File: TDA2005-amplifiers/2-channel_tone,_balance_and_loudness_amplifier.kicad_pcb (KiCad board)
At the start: 2 copper layers, 38 parts, among them U1 TDA2005

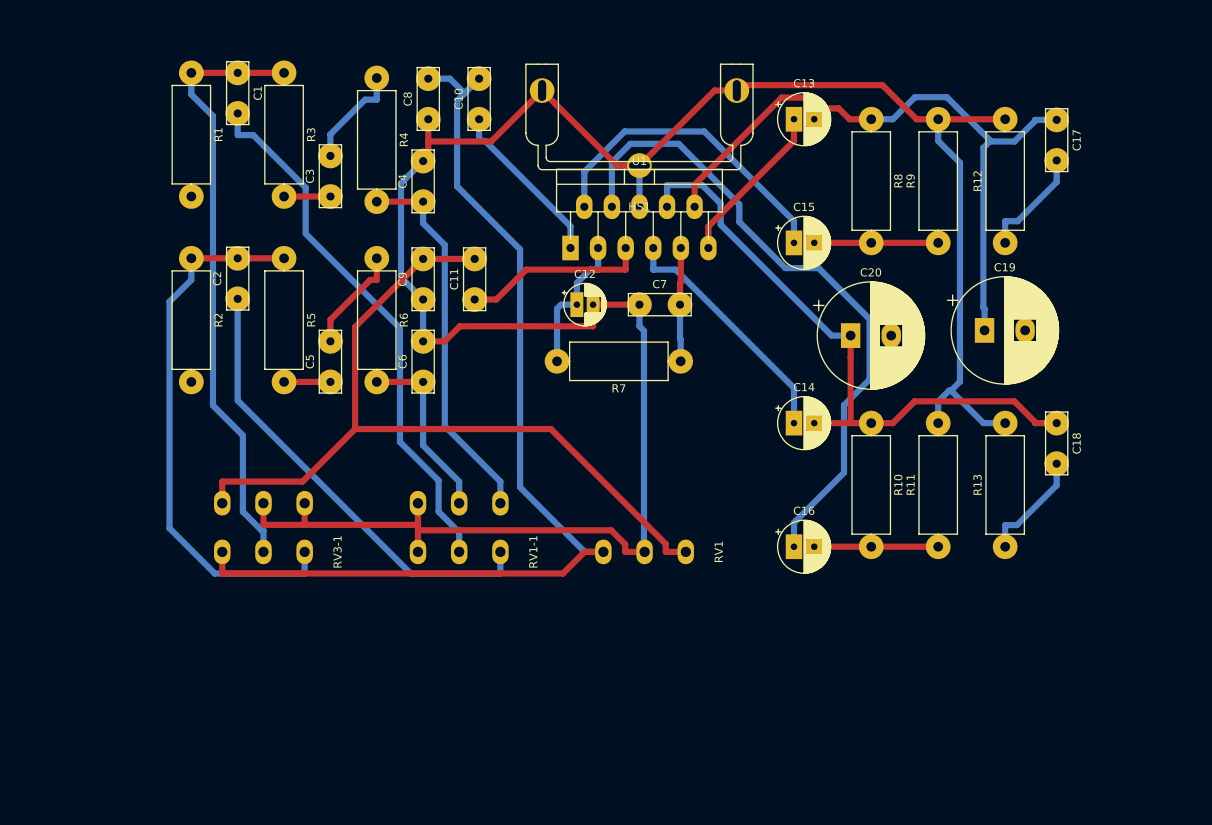
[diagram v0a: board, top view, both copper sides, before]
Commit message: new layout
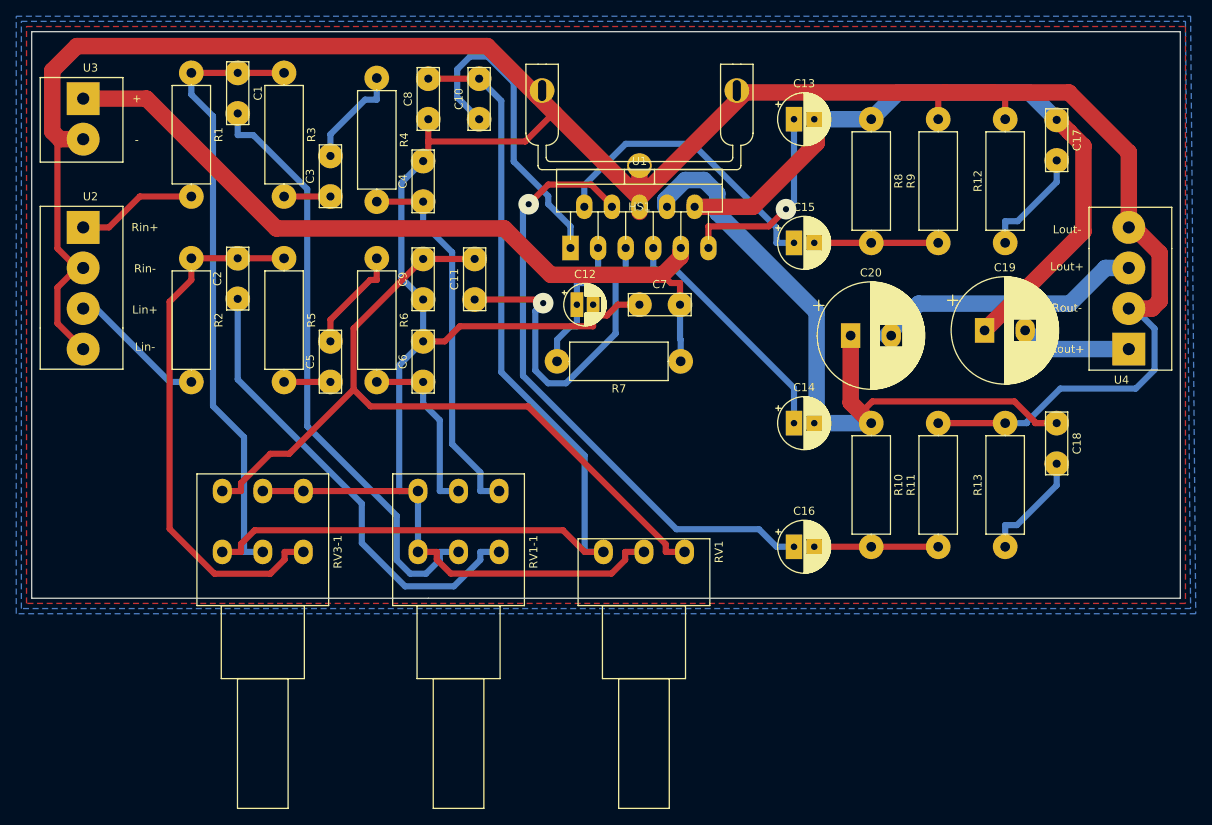
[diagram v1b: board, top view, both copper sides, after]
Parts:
- added U2: 4-pole_RL-input_screw_terminal, My_Parts:4-pole_screw_terminal_RL_input, F.Cu at (111.1, 54.6)
- added U3: 2-pole_power_in_screw_terminal, My_Parts:2-pole_power_in_screw_terminal, F.Cu at (111.1, 38.7)
- added U4: 4-pole_RL-output_screw_terminal, My_Parts:4-pole_screw_terminal_RL_output, F.Cu at (240.0, 69.6)
- RV1: footprint My_Parts:Potentiometer_single_EK#40910007_10k -> My_Misc:Potentiometer_Piher_PC-16_Single_Horizontal_larger
- RV1-1, RV3-1: footprint My_Parts:Potentiometer_double_EK#40910227_10k -> My_Misc:Potentiometer_Piher_PC-16_Dual_Horizontal_larger
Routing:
- net GND: track 287.3 -> 428.4 mm
- net +15V: track 14.0 -> 97.5 mm
- net Lout+: track 0.00 -> 33.9 mm
- net Net-(C11-Pad1): track 22.8 -> 41.5 mm, vias 0 -> 1
- net Net-(C10-Pad1): track 21.0 -> 39.5 mm
- net Lin+: track 0.00 -> 17.1 mm
- net Rout+: track 0.00 -> 15.4 mm
- net Rin+: track 0.00 -> 14.9 mm
- net Net-(C14-Pad2): track 77.5 -> 87.6 mm
- net Net-(C1-Pad2): track 66.6 -> 74.3 mm
- net Net-(C13-Pad2): track 83.4 -> 88.9 mm
- net Net-(C13-Pad1): track 20.3 -> 24.6 mm, vias 0 -> 1
- net Net-(C16-Pad1): track 80.3 -> 76.1 mm, vias 0 -> 1
- net Net-(C15-Pad1): track 39.5 -> 36.8 mm
- net Net-(C11-Pad2): track 100.0 -> 97.6 mm
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- added copper zone on B.Cu, net (none)
- added copper zone on B.Cu, net GND
- added copper zone on F.Cu, net GND
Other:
- board outline added: 141.6 x 69.8 mm
- net class 50 added: clearance 0.762, trace_width 1.27, via_dia 2.54, via_drill 0.762

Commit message: kicad6
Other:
- net class 50 removed
- net class Default removed
